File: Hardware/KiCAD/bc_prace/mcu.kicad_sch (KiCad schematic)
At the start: 19 parts, among them J4 Conn_01x05, U1 STM32U575VITxQ

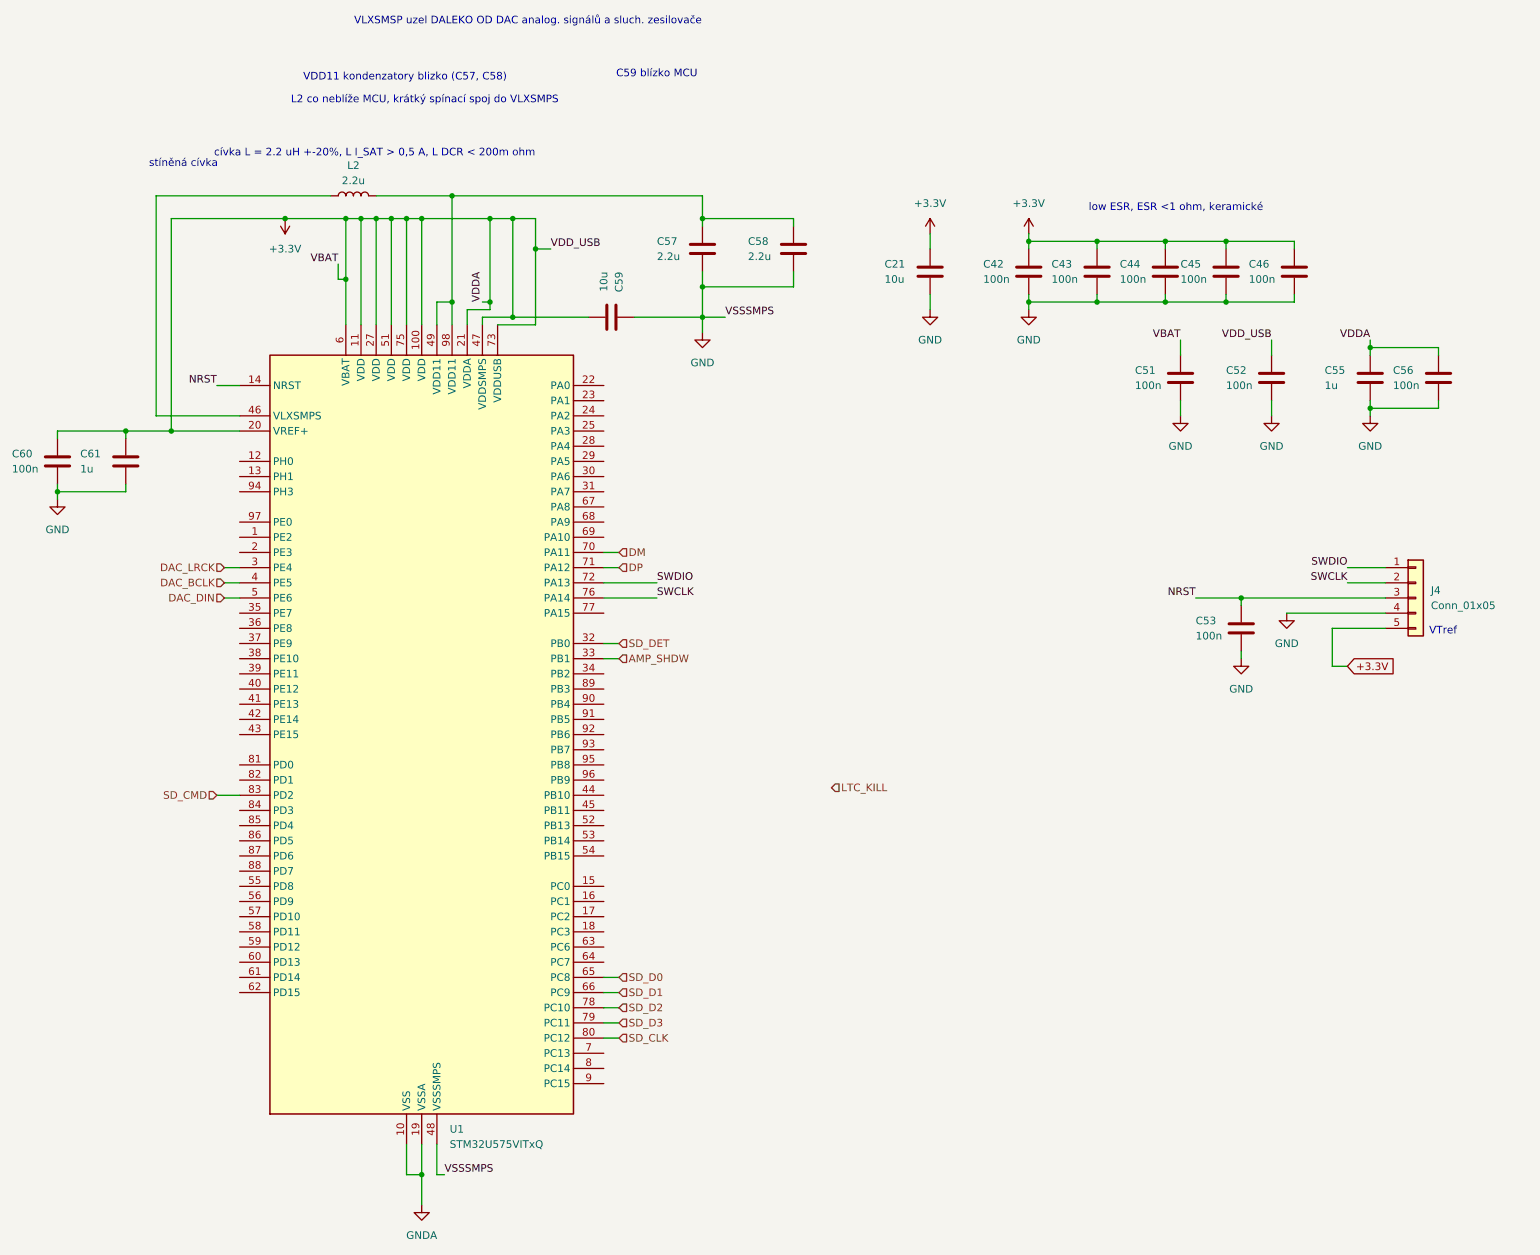
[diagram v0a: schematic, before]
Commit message: ioc, kicad
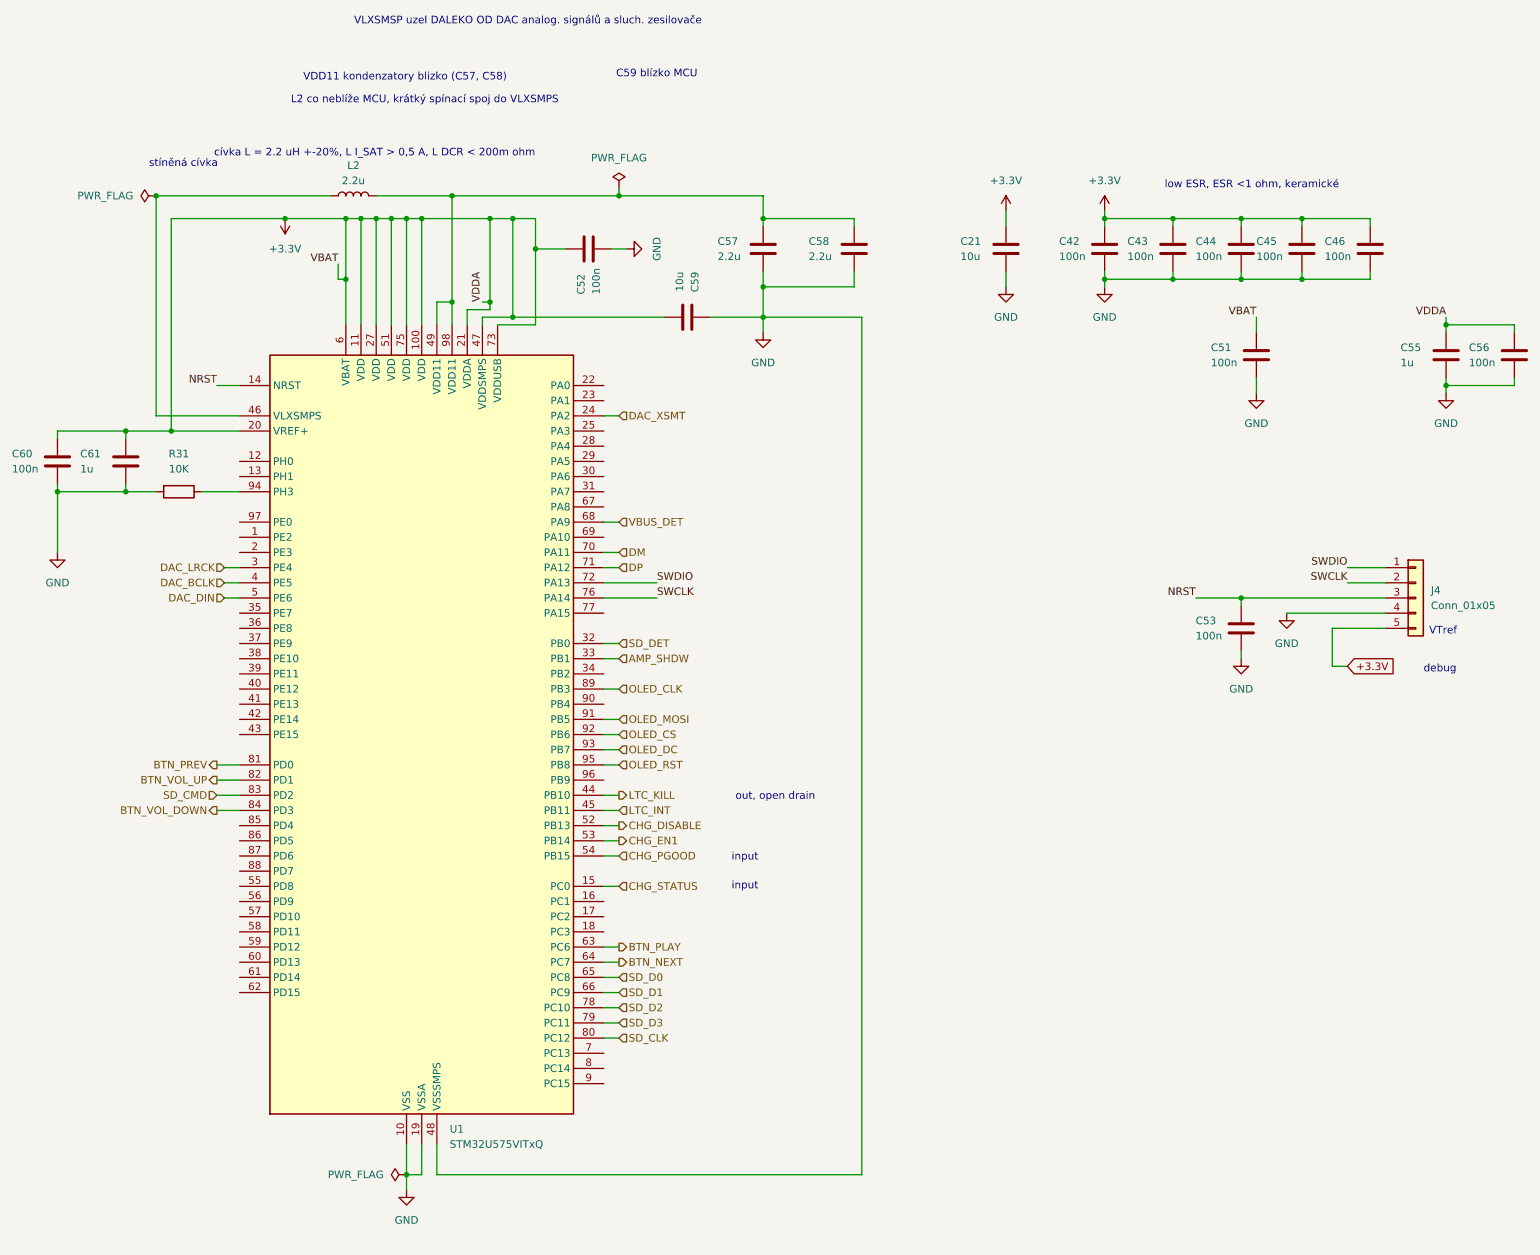
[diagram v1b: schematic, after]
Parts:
- added R31: 10K, Resistor_SMD:R_0805_2012Metric, symbol Device:R
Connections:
- net GNDA is gone; now on net GND: U1.10 (VSS), U1.19 (VSSA), U1.26 (VSS), U1.50 (VSS), U1.74 (VSS), U1.99 (VSS)
- net GND: now also R31.2
- net LTC_KILL: now also U1.44 (PB10)
- net CHG_STATUS: now reaches U1.15 (PC0)
- net DAC_XSMT: now reaches U1.24 (PA2)
- net LTC_INT: now reaches U1.45 (PB11)
- net CHG_DISABLE: now reaches U1.52 (PB13)
- net CHG_EN1: now reaches U1.53 (PB14)
- net CHG_PGOOD: now reaches U1.54 (PB15)
- net BTN_PLAY: now reaches U1.63 (PC6)
- net BTN_NEXT: now reaches U1.64 (PC7)
- net VBUS_DET: now reaches U1.68 (PA9)
- net BTN_PREV: now reaches U1.81 (PD0)
- net BTN_VOL_UP: now reaches U1.82 (PD1)
- net BTN_VOL_DOWN: now reaches U1.84 (PD3)
- net OLED_CLK: now reaches U1.89 (PB3)
- net OLED_MOSI: now reaches U1.91 (PB5)
- net OLED_CS: now reaches U1.92 (PB6)
- net OLED_DC: now reaches U1.93 (PB7)
- net at U1.94 (PH3): now also R31.1
- net OLED_RST: now reaches U1.95 (PB8)
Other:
- note added: "debug"
- note added: "input"
- note added: "out, open drain"
- moved on the sheet: C21, C42, C43, C44, C45, C46, C51, C52, C55, C56, C57, C58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
